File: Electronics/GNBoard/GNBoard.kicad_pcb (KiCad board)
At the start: 2 copper layers, 80 x 55.9 mm, 56 parts, among them K1 IR1, K10 IR4, K11 CNY_1, K12 CNY_2, K13 CNY_3, K14 CNY_4, K17 Nose, K2 IR2, K3 SERVO_1, K4 SERVO_2, K5 SERVO_3, K6 SERVO_4, K7 SERVO_5, K8 SERVO_6, K9 IR3, M1 XBEE, P1 Battery, P2 LDR_1, P3 Spk, P4 I2C_1, P5 LDR_2, P6 DHT_Conn, P7 LDR_3, P8 LDR_4, SW1 PowerSwitch, SW2 SW_PUSH, SW3 SW_PUSH, U1 LM2576

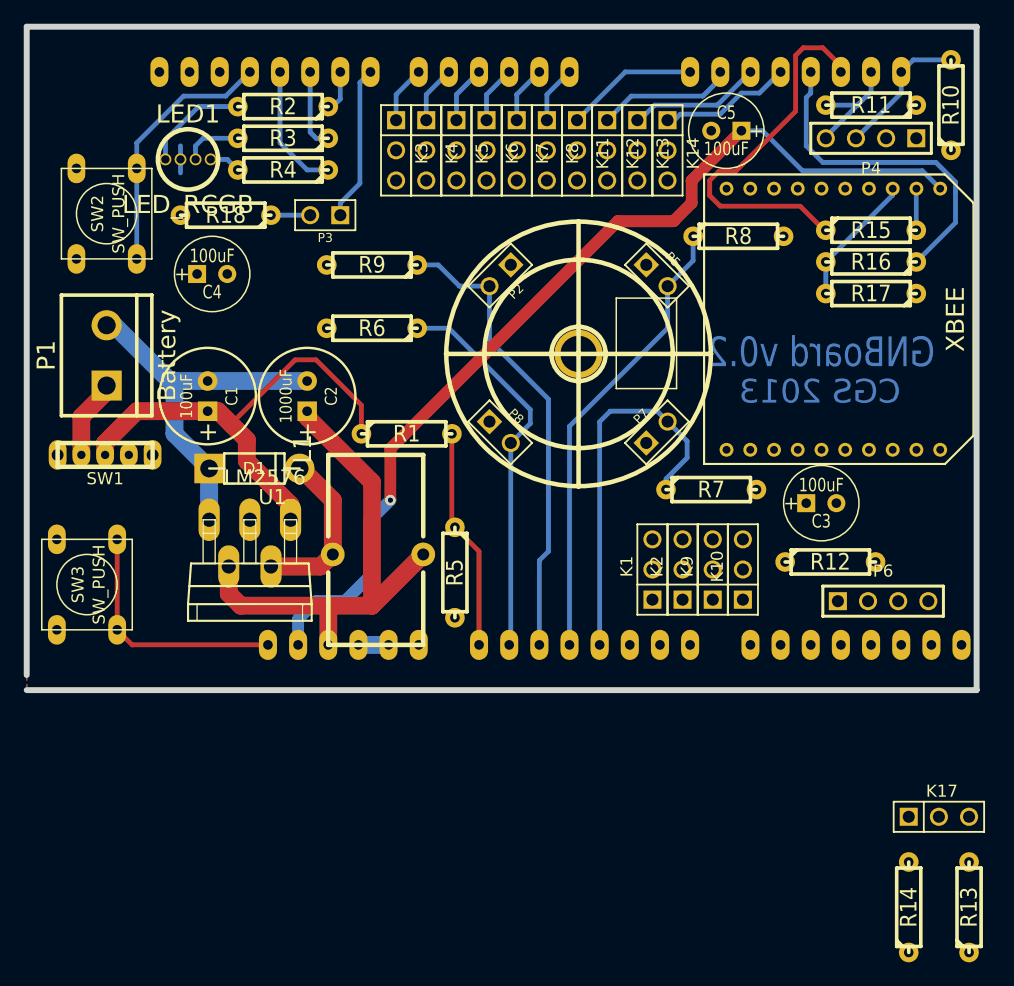
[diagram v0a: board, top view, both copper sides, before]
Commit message: Finished preliminary design
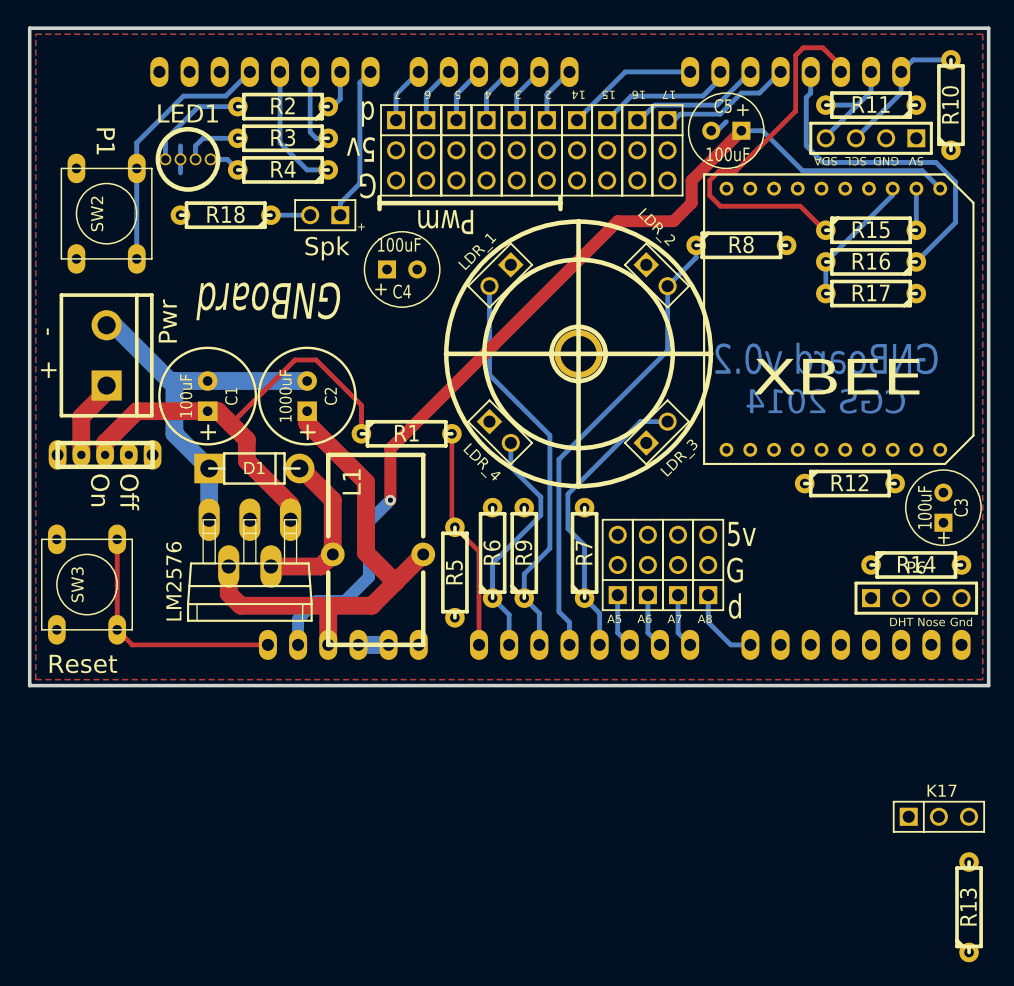
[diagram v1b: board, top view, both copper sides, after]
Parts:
- P1: value Battery -> Pwr
- SHIELD1: footprint ARDUINO_MEGA_SHIELD_MOD -> ARDUINO_MEGA_SHIELD_040pins_MOD
- moved R14 28.8 mm to (124.0, 71.6), turned to 0 degrees
- moved R9 27.4 mm to (90.9, 70.6), turned to 90 degrees
- moved R6 21.5 mm to (88.3, 70.6), turned to 90 degrees
- moved C4 16.0 mm to (80.6, 46.7)
- moved R7 11.9 mm to (96.0, 70.6), turned to 90 degrees
- moved C3 10.3 mm to (126.2, 66.8), turned to 90 degrees
- moved R12 6.81 mm to (118.4, 64.8)
- moved K1 2.95 mm to (98.8, 71.6)
- moved K9 2.95 mm to (103.9, 71.6)
- moved K10 2.95 mm to (106.4, 71.6)
- moved K2 2.95 mm to (101.3, 71.6)
- moved P6 2.81 mm to (124.0, 74.4)
- moved R8 0.80 mm to (109.2, 44.7)
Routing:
- net LDR4: track 32.9 -> 20.3 mm
- net LDR3: track 32.4 -> 24.7 mm
- net V_IR4: track 0.00 -> 6.63 mm
- net LDR1: track 39.4 -> 33.7 mm
- net V_IR3: track 0.00 -> 4.61 mm
- net V_IR1: track 0.00 -> 4.61 mm
- net V_IR2: track 0.00 -> 4.61 mm
- net GND: track 36.9 -> 38.5 mm
- net +5V: track 43.3 -> 42.2 mm
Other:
- board size 80 x 55.9 mm -> 80.8 x 55.4 mm
- board text added: "+"
- board text added: "- +"
- board text added: "14"
- board text added: "15"
- board text added: "16"
- board text added: "17"
- board text added: "2"
- board text added: "3"
- board text added: "4"
- board text added: "5"
- board text added: "5V"
- board text added: "5v"
- board text added: "6"
- board text added: "7"
- board text added: "A5"
- board text added: "A6"
- board text added: "A7"
- board text added: "A8"
- board text added: "CGS 2014"
- board text added: "DHT"
- board text added: "G"
- board text added: "GNBoard"
- board text added: "GND"
- board text added: "Gnd"
- board text added: "Nose"
- board text added: "Off On"
- board text added: "P1"
- board text added: "Pwm"
- board text added: "Reset"
- board text added: "SCL"
- board text added: "SDA"
- board text added: "d"
- board text removed: "CGS 2013"
